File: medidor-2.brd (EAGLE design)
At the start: 31 parts

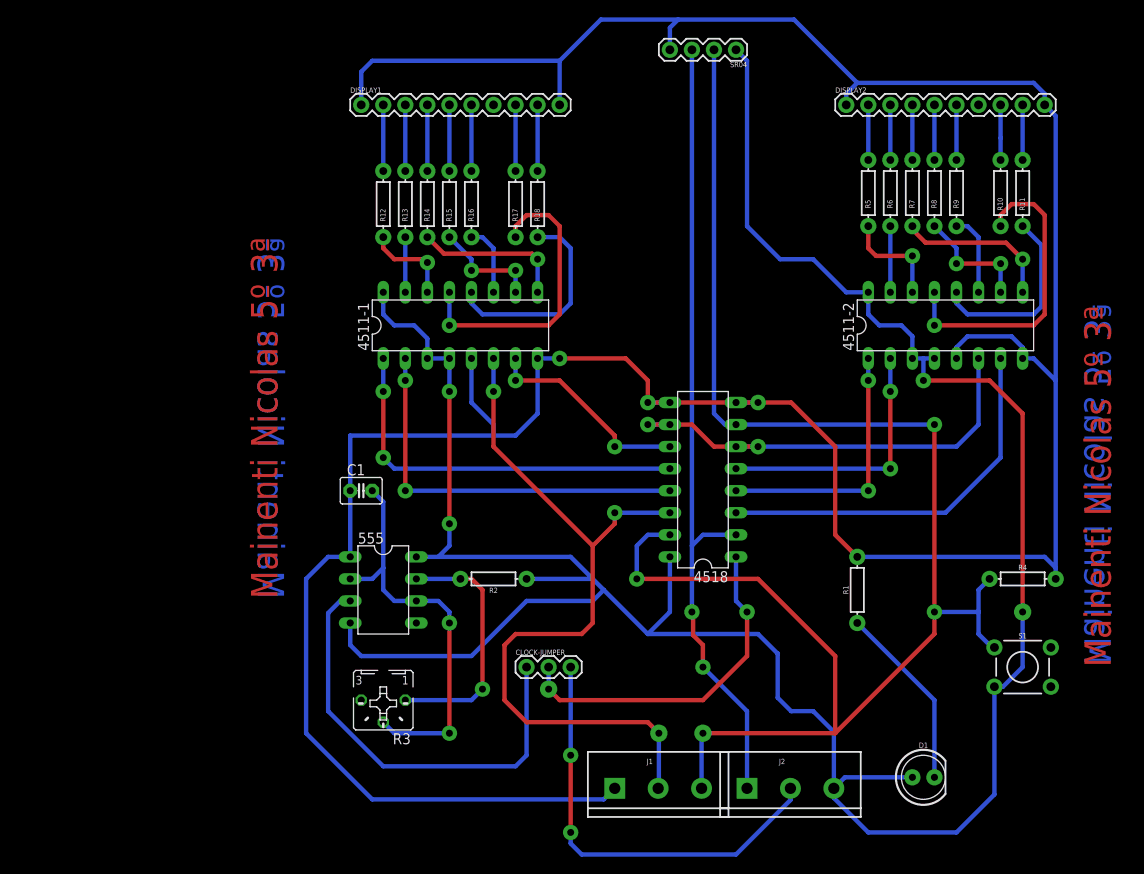
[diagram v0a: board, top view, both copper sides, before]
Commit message: flatcam
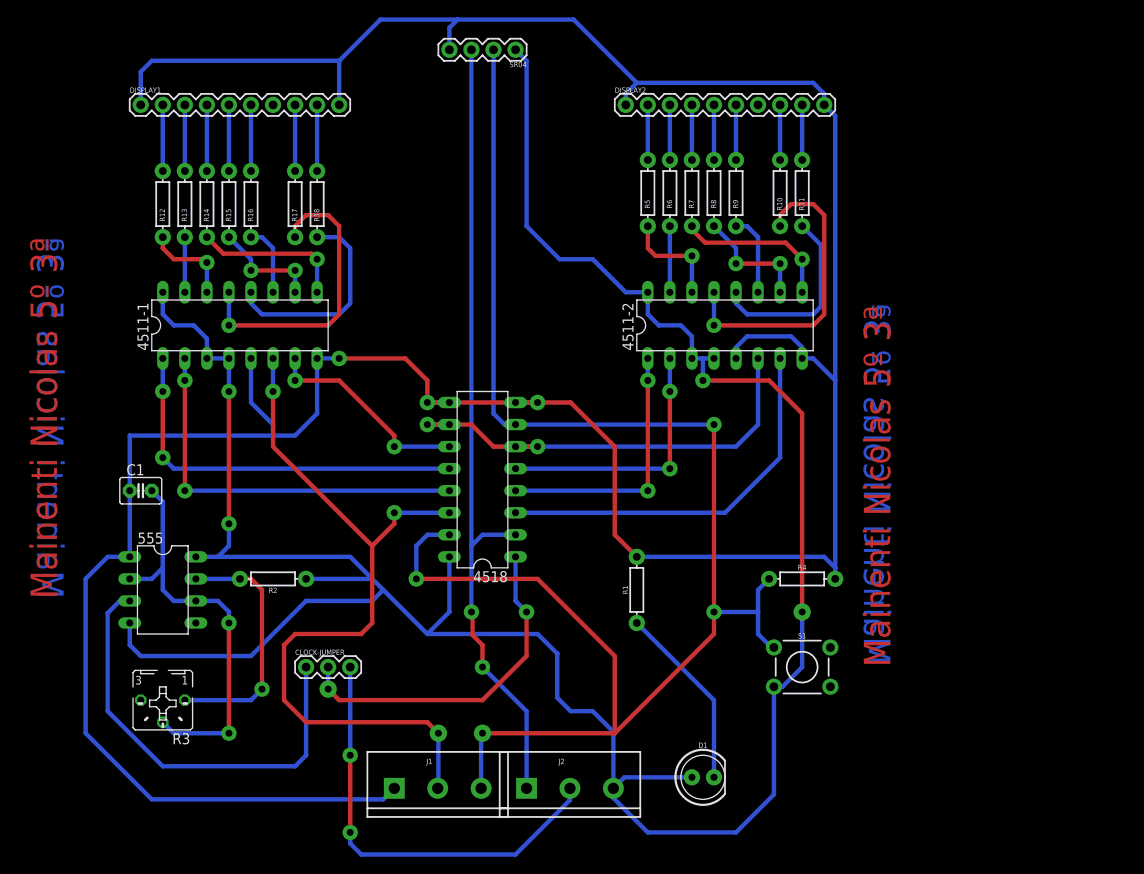
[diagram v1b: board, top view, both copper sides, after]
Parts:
- moved 4511-2 25.4 mm to (82.5, 63.5)
- moved 4518 25.4 mm to (54.6, 45.7)
- moved J2 25.4 mm to (59.7, 10.2)
- moved R1 25.4 mm to (72.4, 33.0)
- moved R11 25.4 mm to (91.4, 78.7)
- moved R4 25.4 mm to (91.4, 34.3)
- moved R5 25.4 mm to (73.7, 78.7)
- moved R7 25.4 mm to (78.7, 78.7)
- moved R8 25.4 mm to (81.3, 78.7)
- moved R9 25.4 mm to (83.8, 78.7)
- moved S1 25.4 mm to (91.4, 24.1)
- moved R16 25.4 mm to (27.9, 77.5)
- moved R2 25.4 mm to (30.5, 34.3)
- moved 4511-1 25.4 mm to (26.7, 63.5)
- moved 555 25.4 mm to (17.8, 33.0)
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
